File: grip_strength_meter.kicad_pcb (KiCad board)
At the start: 2 copper layers, 80 x 40 mm, 0 parts

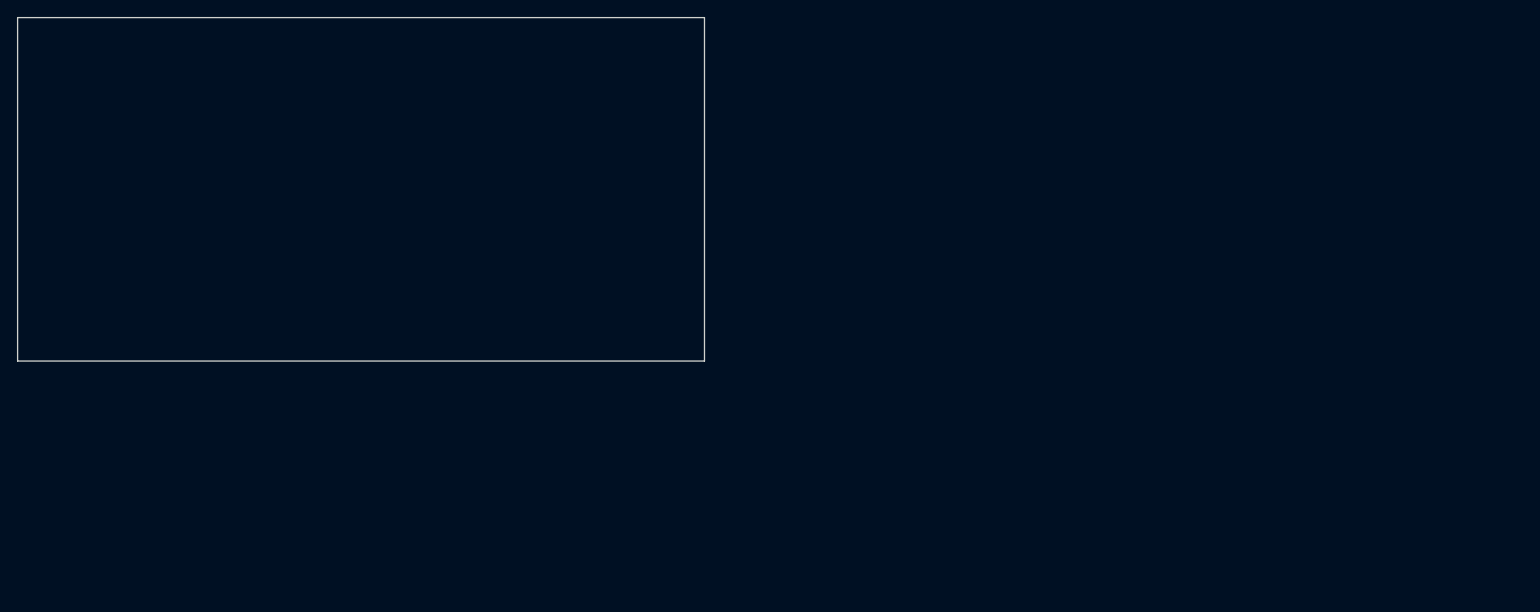
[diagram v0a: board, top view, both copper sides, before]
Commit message: pre pre production
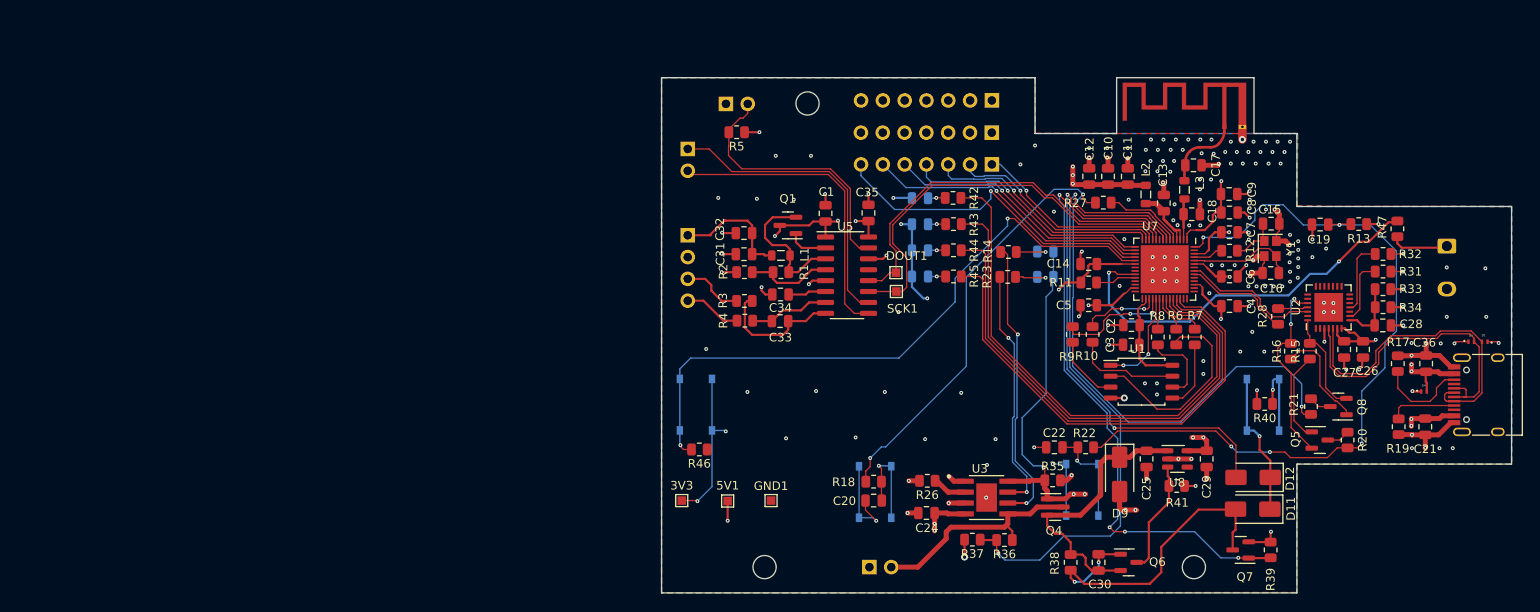
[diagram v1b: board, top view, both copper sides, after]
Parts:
- added 3V3: TestPoint, TestPoint:TestPoint_Pad_1.0x1.0mm, F.Cu at (152.3, 131.2)
- added 5V1: TestPoint, TestPoint:TestPoint_Pad_1.0x1.0mm, F.Cu at (157.7, 131.3)
- added AE2: Antenna_Chip, RF_Antenna:Texas_SWRA117D_2.4GHz_Left, F.Cu at (215.6, 87.7)
- added BAT1: Conn_01x02_Pin, Connector_PinHeader_2.54mm:PinHeader_1x02_P2.54mm_Vertical, B.Cu at (174.2, 139.0)
- added C1: 100nF, Capacitor_SMD:C_0805_2012Metric, F.Cu at (169.1, 97.8)
- added C10: 1uF, Capacitor_SMD:C_0805_2012Metric, F.Cu at (202.0, 93.5)
- added C11: 100nF, Capacitor_SMD:C_0805_2012Metric, F.Cu at (204.3, 93.5)
- added C12: 10uF, Capacitor_SMD:C_0805_2012Metric, F.Cu at (199.8, 93.5)
- added C13: 100nF, Capacitor_SMD:C_0805_2012Metric, F.Cu at (208.5, 96.6)
- added C14: 100nF, Capacitor_SMD:C_0805_2012Metric, F.Cu at (199.8, 103.7)
- added C15: 10pF, Capacitor_SMD:C_0805_2012Metric, F.Cu at (221.0, 99.0)
- added C16: 10pF, Capacitor_SMD:C_0805_2012Metric, F.Cu at (220.9, 104.8)
- added C17: 10pF, Capacitor_SMD:C_0805_2012Metric, F.Cu at (211.9, 92.2)
- added C18: 10pF, Capacitor_SMD:C_0805_2012Metric, F.Cu at (211.8, 97.9)
- added C19: 1uF, Capacitor_SMD:C_0805_2012Metric, F.Cu at (226.7, 99.1)
- added C2: 100nF, Capacitor_SMD:C_0805_2012Metric, F.Cu at (204.7, 110.8)
- added C20: 100 nF, Capacitor_SMD:C_0805_2012Metric, F.Cu at (174.7, 131.2)
- added C21: 5uF, Capacitor_SMD:C_0805_2012Metric, F.Cu at (238.9, 122.7)
- added C22: 100 nF, Capacitor_SMD:C_0805_2012Metric, F.Cu at (195.8, 125.0)
- added C24: 10uF, Capacitor_SMD:C_0805_2012Metric, F.Cu at (180.8, 132.7)
- added C25: 2uF, Capacitor_SMD:C_0805_2012Metric, F.Cu at (206.5, 126.4)
- added C26: 100nF, Capacitor_SMD:C_0805_2012Metric, F.Cu at (231.7, 113.7)
- added C27: 4.7uF, Capacitor_SMD:C_0805_2012Metric, F.Cu at (229.5, 113.7)
- added C28: 10uF, Capacitor_SMD:C_0805_2012Metric, F.Cu at (234.0, 110.8)
- added C29: 2uF, Capacitor_SMD:C_0805_2012Metric, F.Cu at (213.5, 126.4)
- added C3: 1uF, Capacitor_SMD:C_0805_2012Metric, F.Cu at (204.7, 113.1)
- added C30: 100n, Capacitor_SMD:C_0805_2012Metric, F.Cu at (200.9, 138.4)
- added C31: 100nF, Capacitor_SMD:C_0805_2012Metric, F.Cu at (159.6, 102.5)
- added C32: 10uF, Capacitor_SMD:C_0805_2012Metric, F.Cu at (159.6, 100.1)
- added C33: 100nF, Capacitor_SMD:C_0805_2012Metric, F.Cu at (163.8, 110.3)
- added C34: 100nF, Capacitor_SMD:C_0805_2012Metric, F.Cu at (163.8, 107.2)
- added C35: 10uF, Capacitor_SMD:C_0805_2012Metric, F.Cu at (174.1, 97.8)
- added C36: 5uF, Capacitor_SMD:C_0805_2012Metric, F.Cu at (239.1, 115.3)
- added C4: 100nF, Capacitor_SMD:C_0805_2012Metric, F.Cu at (216.2, 108.6)
- added C5: 100nF, Capacitor_SMD:C_0805_2012Metric, F.Cu at (199.8, 108.5)
- added C6: 100nF, Capacitor_SMD:C_0805_2012Metric, F.Cu at (216.2, 105.2)
- added C7: 100nF, Capacitor_SMD:C_0805_2012Metric, F.Cu at (216.2, 100.0)
- added C8: 100nF, Capacitor_SMD:C_0805_2012Metric, F.Cu at (216.2, 97.7)
- added C9: 1uF, Capacitor_SMD:C_0805_2012Metric, F.Cu at (216.1, 95.5)
- added D1: H5VL10B, PMEG2005AEL_315:DIODFN2_98X58X50L26X51N, F.Cu at (245.9, 112.8)
- added D11: SS54, Diode_SMD:D_SMA, F.Cu at (218.8, 132.2)
- added D12: SS54, Diode_SMD:D_SMA, F.Cu at (218.9, 128.6)
- added D13: LED, LED_SMD:LED_0805_2012Metric, B.Cu at (180.1, 96.0)
- added D14: LED, LED_SMD:LED_0805_2012Metric, B.Cu at (180.1, 99.1)
- added D15: LED, LED_SMD:LED_0805_2012Metric, B.Cu at (180.1, 102.1)
- added D16: LED, LED_SMD:LED_0805_2012Metric, B.Cu at (180.1, 105.2)
- added D3: H5VL10B, PMEG2005AEL_315:DIODFN2_98X58X50L26X51N, F.Cu at (244.3, 112.8)
- added D4: H5VL10B, PMEG2005AEL_315:DIODFN2_98X58X50L26X51N, F.Cu at (238.8, 118.5)
- added D7: RED LED, LED_SMD:LED_0805_2012Metric, B.Cu at (194.7, 105.2)
- added D8: GREEN LED, LED_SMD:LED_0805_2012Metric, B.Cu at (194.7, 102.2)
- added D9: SS54, Diode_SMD:D_SMA, F.Cu at (203.3, 128.2)
- added DOUT1: TestPoint, TestPoint:TestPoint_Pad_1.0x1.0mm, F.Cu at (177.3, 104.7)
- added GND1: TestPoint, TestPoint:TestPoint_Pad_1.0x1.0mm, F.Cu at (162.8, 131.2)
- added H1: MountingHole, MountingHole:MountingHole_2.7mm_M2.5_ISO7380, F.Cu at (167.0, 85.0)
- added H2: MountingHole, MountingHole:MountingHole_2.7mm_M2.5_ISO7380, F.Cu at (212.0, 139.0)
- added H3: MountingHole, MountingHole:MountingHole_2.7mm_M2.5_ISO7380, F.Cu at (162.0, 139.0)
- added J1: Conn_01x04_Male, Connector_PinHeader_2.54mm:PinHeader_1x04_P2.54mm_Vertical, B.Cu at (153.1, 100.3)
- added J2: Conn_01x02_Male, Connector_PinHeader_2.54mm:PinHeader_1x02_P2.54mm_Vertical, B.Cu at (153.1, 90.3)
- added J3: Conn_01x02_Male, Connector_PinHeader_2.54mm:PinHeader_1x02_P2.54mm_Vertical, B.Cu at (157.5, 85.0)
- added J4: Conn_01x07_Pin, Connector_PinHeader_2.54mm:PinHeader_1x07_P2.54mm_Vertical, B.Cu at (188.5, 92.1)
- added J5: Conn_01x07_Pin, Connector_PinHeader_2.54mm:PinHeader_1x07_P2.54mm_Vertical, B.Cu at (188.5, 84.7)
- added J6: Conn_01x07_Pin, Connector_PinHeader_2.54mm:PinHeader_1x07_P2.54mm_Vertical, B.Cu at (188.5, 88.4)
- added L1: 3.3uH, Inductor_SMD:L_0805_2012Metric, F.Cu at (163.9, 102.7)
- added L2: 2nH, Inductor_SMD:L_0805_2012Metric, F.Cu at (206.4, 95.6)
- added L3: 2nH, Inductor_SMD:L_0805_2012Metric, F.Cu at (210.9, 95.1)
- added OUTPUT1: Screw_Terminal_01x02, screws:screw-2-pin, B.Cu at (246.5, 104.2)
- added Q1: SS8550, Package_TO_SOT_SMD:SOT-23, F.Cu at (164.7, 99.2)
- added Q4: AO3401A, Package_TO_SOT_SMD:SOT-23, F.Cu at (195.8, 132.0)
- added Q5: MMBT3904, Package_TO_SOT_SMD:SOT-23, F.Cu at (226.7, 124.2)
- added Q6: AO3401A, Package_TO_SOT_SMD:SOT-23, F.Cu at (204.4, 138.4)
- added Q7: AO3400A, Package_TO_SOT_SMD:SOT-23, F.Cu at (217.4, 137.0)
- added Q8: MMBT3904, Package_TO_SOT_SMD:SOT-23, F.Cu at (228.8, 120.3)
- added R1: 20K, Resistor_SMD:R_0805_2012Metric, F.Cu at (163.9, 104.7)
- added R10: 0R, Resistor_SMD:R_0805_2012Metric, F.Cu at (200.2, 111.9)
- added R11: 10K, Resistor_SMD:R_0805_2012Metric, F.Cu at (199.8, 105.8)
- added R12: 0R, Resistor_SMD:R_0805_2012Metric, F.Cu at (216.2, 102.2)
- added R13: 10K, Resistor_SMD:R_0805_2012Metric, F.Cu at (231.2, 99.0)
- added R14: 1K, Resistor_SMD:R_0805_2012Metric, F.Cu at (190.4, 102.3)
- added R15: 10K, Resistor_SMD:R_0805_2012Metric, F.Cu at (225.5, 113.8)
- added R16: 10K, Resistor_SMD:R_0805_2012Metric, F.Cu at (223.3, 113.8)
- added R17: 5K1, Resistor_SMD:R_0805_2012Metric, F.Cu at (235.8, 115.3)
- added R18: 0R, Resistor_SMD:R_0805_2012Metric, F.Cu at (174.7, 129.1)
- added R19: 5K1, Resistor_SMD:R_0805_2012Metric, F.Cu at (235.8, 122.7)
- added R2: 8.2K, Resistor_SMD:R_0805_2012Metric, F.Cu at (159.7, 104.7)
- added R20: 0R, Resistor_SMD:R_0805_2012Metric, F.Cu at (229.9, 124.2)
- added R21: 0R, Resistor_SMD:R_0805_2012Metric, F.Cu at (225.6, 120.3)
- added R22: 0R, Resistor_SMD:R_0805_2012Metric, F.Cu at (199.4, 125.0)
- added R23: 1K, Resistor_SMD:R_0805_2012Metric, F.Cu at (190.3, 105.2)
- added R26: 1K5, Resistor_SMD:R_0805_2012Metric, F.Cu at (180.9, 128.9)
- added R27: 22R, Resistor_SMD:R_0805_2012Metric, F.Cu at (201.4, 96.5)
- added R28: 499R, Resistor_SMD:R_0805_2012Metric, F.Cu at (221.8, 109.8)
- added R3: 100R, Resistor_SMD:R_0805_2012Metric, F.Cu at (159.7, 108.0)
- added R31: 4K7, Resistor_SMD:R_0805_2012Metric, F.Cu at (234.0, 104.6)
- added R32: 10K, Resistor_SMD:R_0805_2012Metric, F.Cu at (234.0, 102.5)
- added R33: 24K, Resistor_SMD:R_0805_2012Metric, F.Cu at (234.0, 106.6)
- added R34: 47K, Resistor_SMD:R_0805_2012Metric, F.Cu at (234.0, 108.7)
- added R35: 100K, Resistor_SMD:R_0805_2012Metric, F.Cu at (195.6, 128.9)
- added R36: 10K, Resistor_SMD:R_0805_2012Metric, F.Cu at (189.9, 135.8)
- added R37: 30K, Resistor_SMD:R_0805_2012Metric, F.Cu at (186.2, 135.8)
- added R38: 100K, Resistor_SMD:R_0805_2012Metric, F.Cu at (197.7, 138.4)
- added R39: 1M, Resistor_SMD:R_0805_2012Metric, F.Cu at (220.9, 137.0)
- added R4: 100R, Resistor_SMD:R_0805_2012Metric, F.Cu at (159.7, 110.3)
- added R40: 100R, Resistor_SMD:R_0805_2012Metric, F.Cu at (220.2, 120.0)
- added R41: 100K, Resistor_SMD:R_0805_2012Metric, F.Cu at (210.0, 129.6)
- added R42: 5K, Resistor_SMD:R_0805_2012Metric, F.Cu at (183.9, 96.0)
- added R43: 5K, Resistor_SMD:R_0805_2012Metric, F.Cu at (184.0, 99.0)
- added R44: 5K, Resistor_SMD:R_0805_2012Metric, F.Cu at (184.0, 102.1)
- added R45: 5K, Resistor_SMD:R_0805_2012Metric, F.Cu at (184.0, 105.2)
- added R46: 10K, Resistor_SMD:R_0805_2012Metric, F.Cu at (154.4, 125.3)
- added R47: 0R, Resistor_SMD:R_0805_2012Metric, F.Cu at (235.7, 99.6)
- added R5: 20K, Resistor_SMD:R_0805_2012Metric, F.Cu at (158.8, 88.3)
- added R6: 0R, Resistor_SMD:R_0805_2012Metric, F.Cu at (209.9, 112.2)
- added R7: 0R, Resistor_SMD:R_0805_2012Metric, F.Cu at (212.1, 112.2)
- added R8: 0R, Resistor_SMD:R_0805_2012Metric, F.Cu at (207.8, 112.2)
- added R9: 0R, Resistor_SMD:R_0805_2012Metric, F.Cu at (197.9, 111.9)
- added S1: TS-1187A-B-A-B, TS-1187A-B-A-B:SW_TS-1187A-B-A-B, B.Cu at (174.9, 130.2)
- added S2: TS-1187A-B-A-B, TS-1187A-B-A-B:SW_TS-1187A-B-A-B, B.Cu at (199.0, 130.0)
- added S3: TS-1187A-B-A-B, TS-1187A-B-A-B:SW_TS-1187A-B-A-B, B.Cu at (220.1, 120.1)
- added S4: TS-1187A-B-A-B, TS-1187A-B-A-B:SW_TS-1187A-B-A-B, B.Cu at (154.0, 120.1)
- added SCK1: TestPoint, TestPoint:TestPoint_Pad_1.0x1.0mm, F.Cu at (177.3, 106.9)
- added U1: W25Q128JVS, Package_SO:SOIC-8_5.23x5.23mm_P1.27mm, F.Cu at (205.9, 117.4)
- added U2: CP2102, Package_DFN_QFN:QFN-28-1EP_5x5mm_P0.5mm_EP3.35x3.35mm, F.Cu at (227.7, 108.8)
- added U3: TP4056, TP4056:SOP127P600X175-9N, F.Cu at (187.9, 130.9)
- added U5: HX711, Package_SO:SOP-16_3.9x9.9mm_P1.27mm, F.Cu at (171.6, 105.0)
- added U7: ESP32-S2, Package_DFN_QFN:QFN-56-1EP_7x7mm_P0.4mm_EP5.6x5.6mm, F.Cu at (208.6, 104.3)
- added U8: TLV75733PDBV, Package_TO_SOT_SMD:SOT-23-5, F.Cu at (210.1, 126.4)
- added USBC1: USB_C_Receptacle_USB2.0, Connector_USB:USB_C_Receptacle_HRO_TYPE-C-31-M-12, F.Cu at (246.3, 118.9)
- added Y1: Crystal_GND24, Crystal:Crystal_SMD_2520-4Pin_2.5x2.0mm, F.Cu at (220.9, 101.9)
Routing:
- net /3V3: track 0.00 -> 372.2 mm, vias 0 -> 20
- net /5V_USB: track 0.00 -> 176.7 mm, vias 0 -> 13
- net GND: track 0.00 -> 138.2 mm, vias 0 -> 185
- net /mcu_buttons_leds/CIO0_BTN: track 0.00 -> 107.1 mm, vias 0 -> 3
- net /mcu_buttons_leds/CHIP_EN: track 0.00 -> 89.5 mm, vias 0 -> 5
- net /GPIO_POWEROFF: track 0.00 -> 76.7 mm, vias 0 -> 4
- net /V_BAT_MEASURE: track 0.00 -> 75.2 mm, vias 0 -> 2
- net /mcu_buttons_leds/GPIO14: track 0.00 -> 74.9 mm, vias 0 -> 2
- net Net-(U7-GPIO33): track 0.00 -> 63.6 mm
- net /GPIO_BUTTON_CHECK: track 0.00 -> 62.6 mm, vias 0 -> 2
- net Net-(U7-GPIO34): track 0.00 -> 61.4 mm
- net Net-(U7-GPIO35): track 0.00 -> 59.2 mm
- net Net-(U7-GPIO36): track 0.00 -> 56.9 mm
- net /PD_SCK: track 0.00 -> 47.8 mm
- net /DOUT: track 0.00 -> 45.8 mm
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- added copper zone on B.Cu, net GND
- added copper zone on F.Cu, net GND
- added copper zone on In1.Cu, net GND
- added copper zone on In2.Cu, net GND
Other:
- board size 80 x 40 mm -> 99 x 60 mm
- copper layers 2 -> 4
- board text added: "A+"
- board text added: "A-"
- board text added: "B+"
- board text added: "B-"
- board text added: "BATTERY"
- board text added: "BOOT MODE"
- board text added: "E+"
- board text added: "E-"
- board text added: "GND"
- board text added: "OUT"
- board text added: "POWER"
- board text added: "RESET"
- board text added: "Remove J3 to get HX711 data rate 80 sps, set J3 to get rate 10 sps but lower noise"
- board text added: "SYSTEM"
- board text added: "face to user buttons and leds"
- board text added: "https://docs.espressif.com/projects/esp-hardware-design-guidelines/en/latest/esp32/pcb-layout-design.html"
- board text added: "jlcpcb min free via size 0.45, hole diam 0.2"
